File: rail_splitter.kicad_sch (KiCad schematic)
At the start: 74 parts, among them J1 input +, J2 input -, J3 +load, J4 gnd load, J5 -load, J6 shunt+ display pos, J7 shunt- display pos, J8 shunt+ display neg, J9 shunt- display neg, Q1 PNP, Q11 NMOS, Q2 NPN, Q3 NPN, Q4 dar, Q5 NPN, Q6 PNP, Q7 PMOS, SW1 SW_Push, SW2 SW_DPST, U1 OP07, U2 NE5532, U3 NE5532, U4 NE5532, U5 LM2936-3.3, U6 NE5532

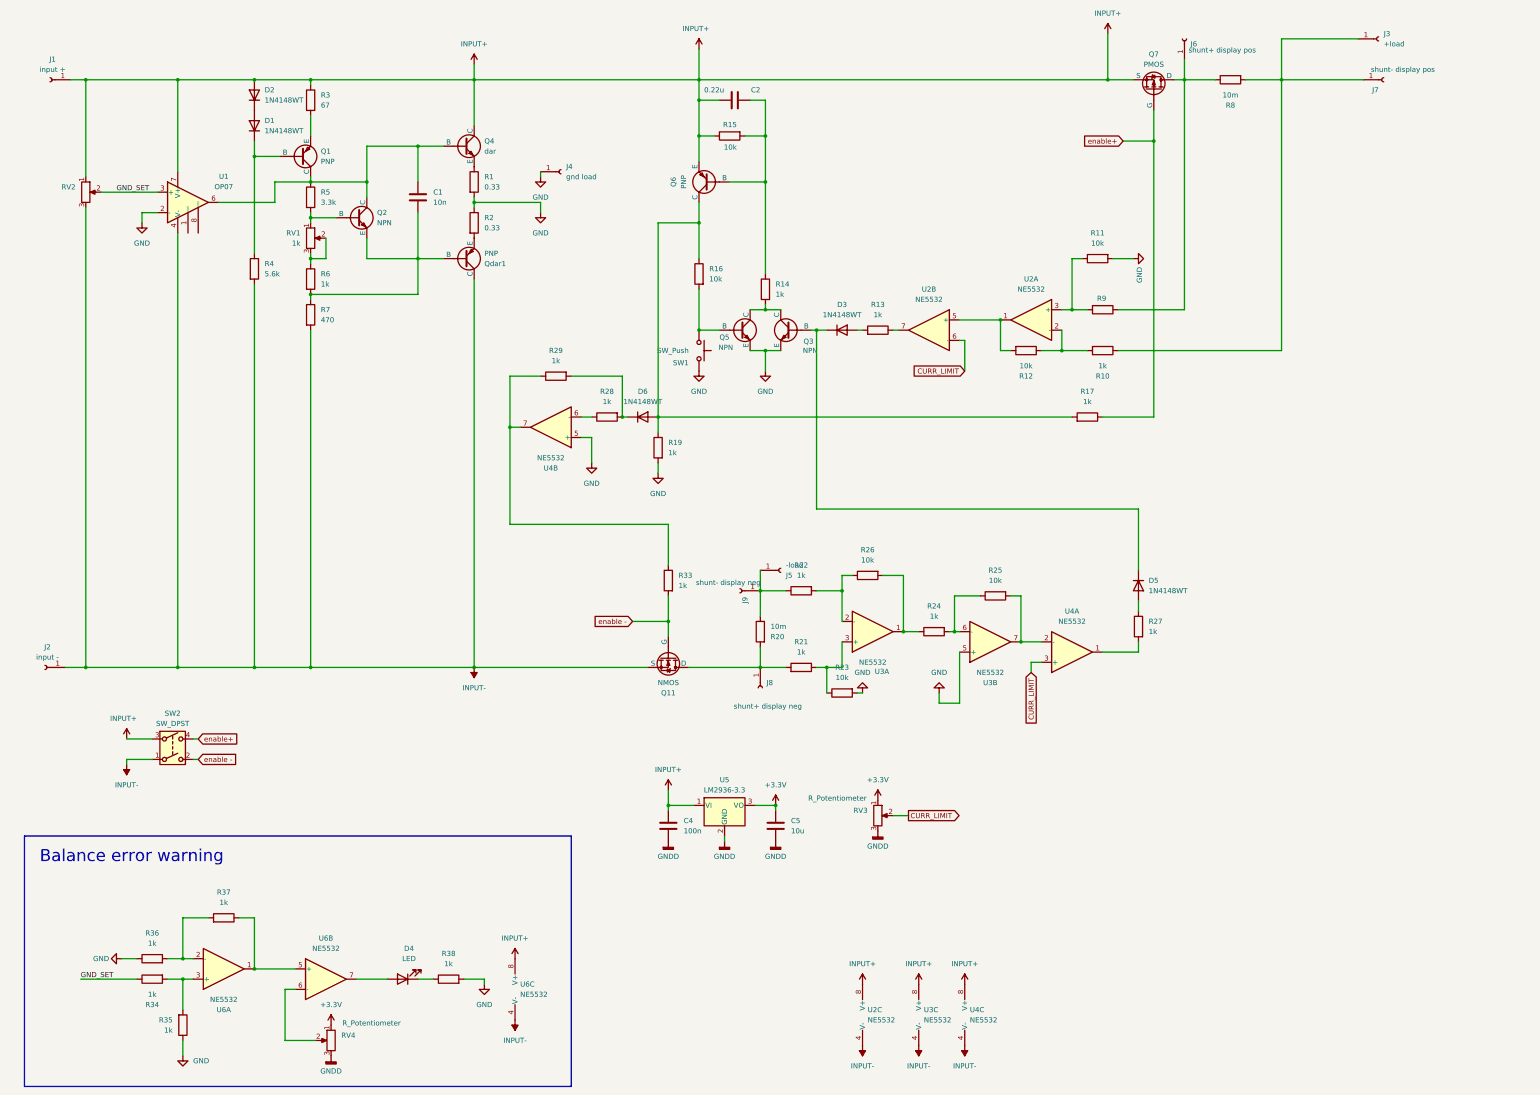
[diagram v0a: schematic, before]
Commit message: korekcija izgleda, more TBD.
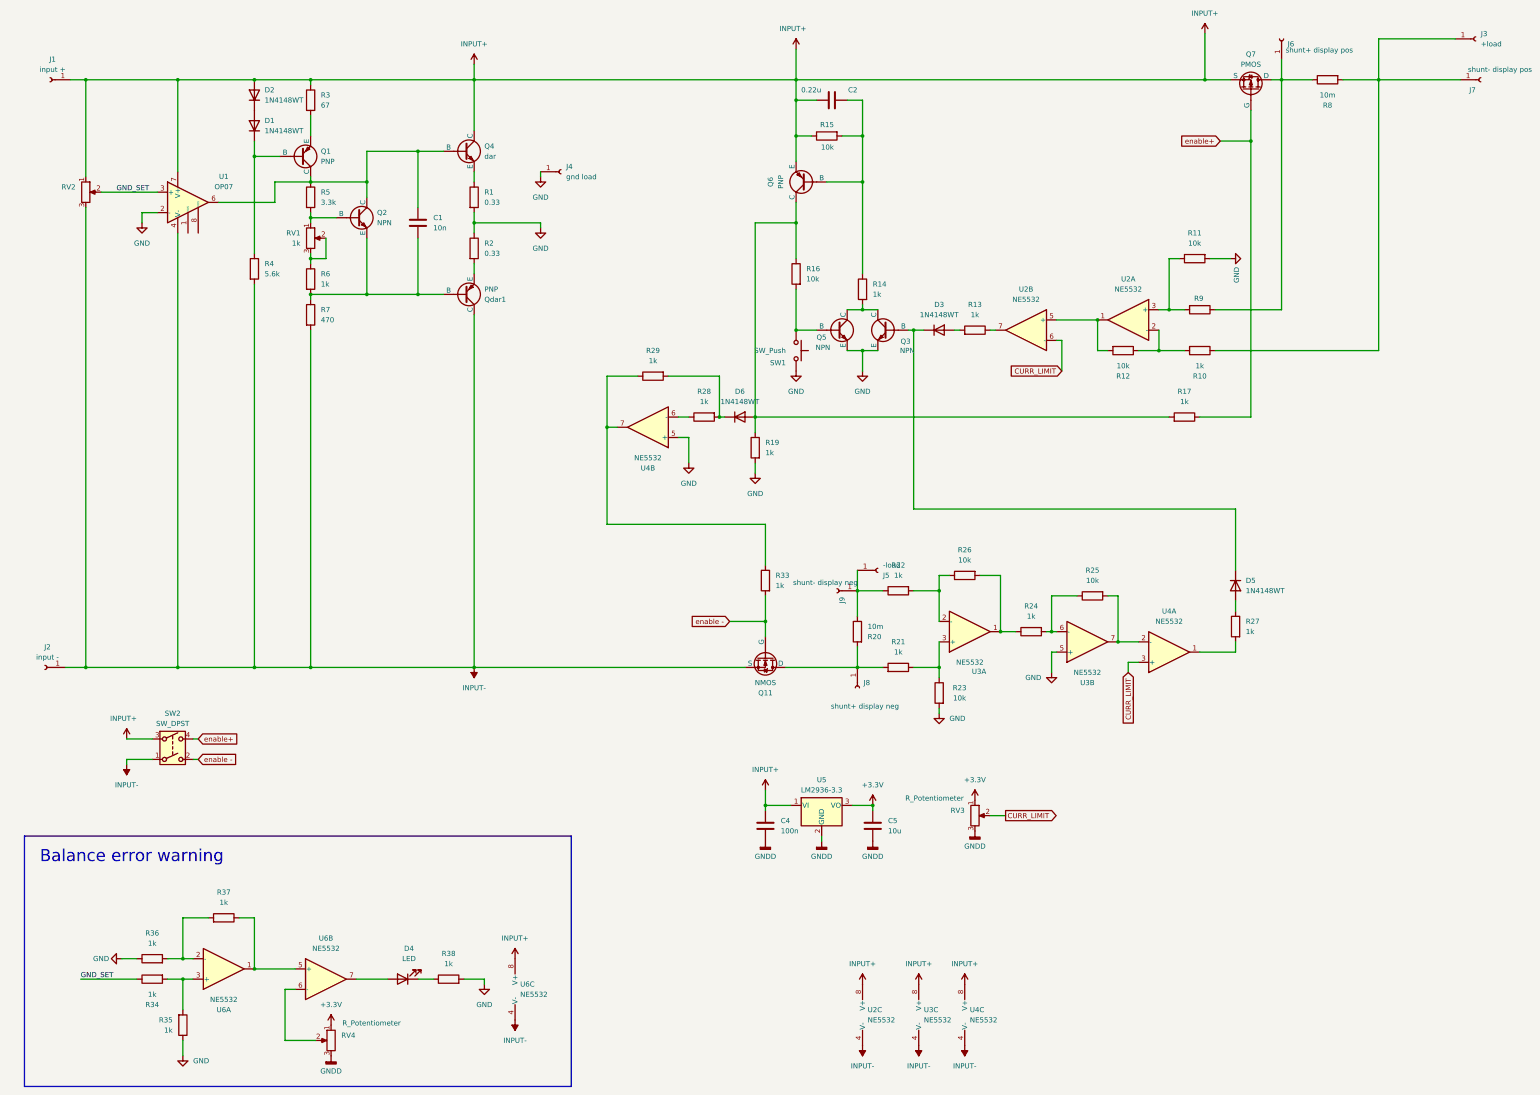
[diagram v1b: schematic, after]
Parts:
- added unit 2 of U4
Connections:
- net GND: now also U4.5 (+); no longer U4.5 (+)
- net at R29.1, R33.1: now also U4.7; no longer U4.7
- net at R28.1: now also U4.6 (-); no longer U4.6 (-)
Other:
- moved on the sheet: C1, C2, C4, C5, D3, D5, D6, J3, J5, J6, J7, J8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
